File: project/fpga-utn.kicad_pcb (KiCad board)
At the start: 2 copper layers, 100 x 75 mm, 144 parts, among them J1 USB_C_Receptacle_USB2.0_16P, P1 Conector SMD 2x10, P2 Conector SMD 2x10, P3 Conector SMD 2x10, P4 Conector SMD 2x10, SW1 SW_Push, SW2 SW_Push, SW3 SW_Push, SW4 SW_Push, SW5 SW_Push, SW6 SW_Push, SW7 SW_Push, SW8 SW_Push, U1 LD1117S33TR_SOT223, U2 LD1117S12TR_SOT223, U3 USBLC6-2SC6, U4 FT2232HL, U5 M93C66, U6 ICE40HX4K-TQ144, U7 W25X40CLSN, Y1 ECS-3225MV-120-CN-TR, Y2 ECS-3225MVQ-1000-CN-TR

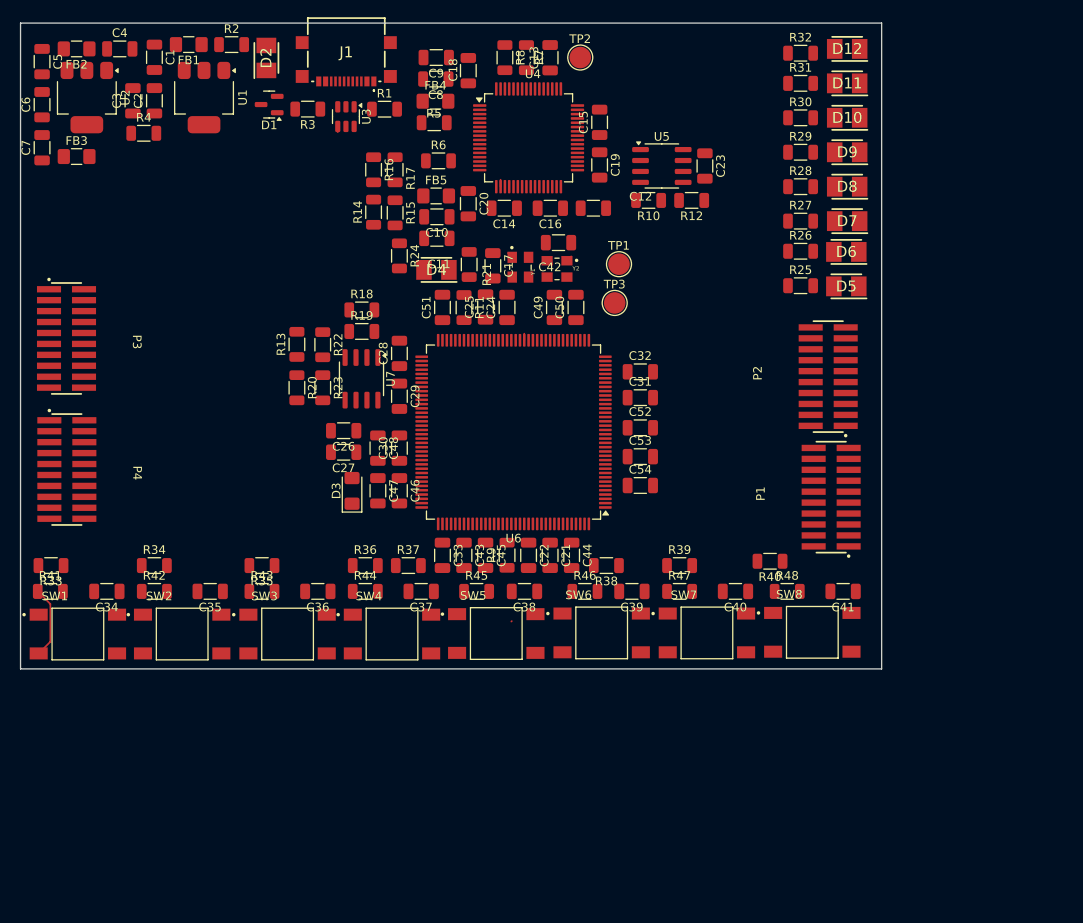
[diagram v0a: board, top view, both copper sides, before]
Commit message: Version 1 pcb, sin finalizar
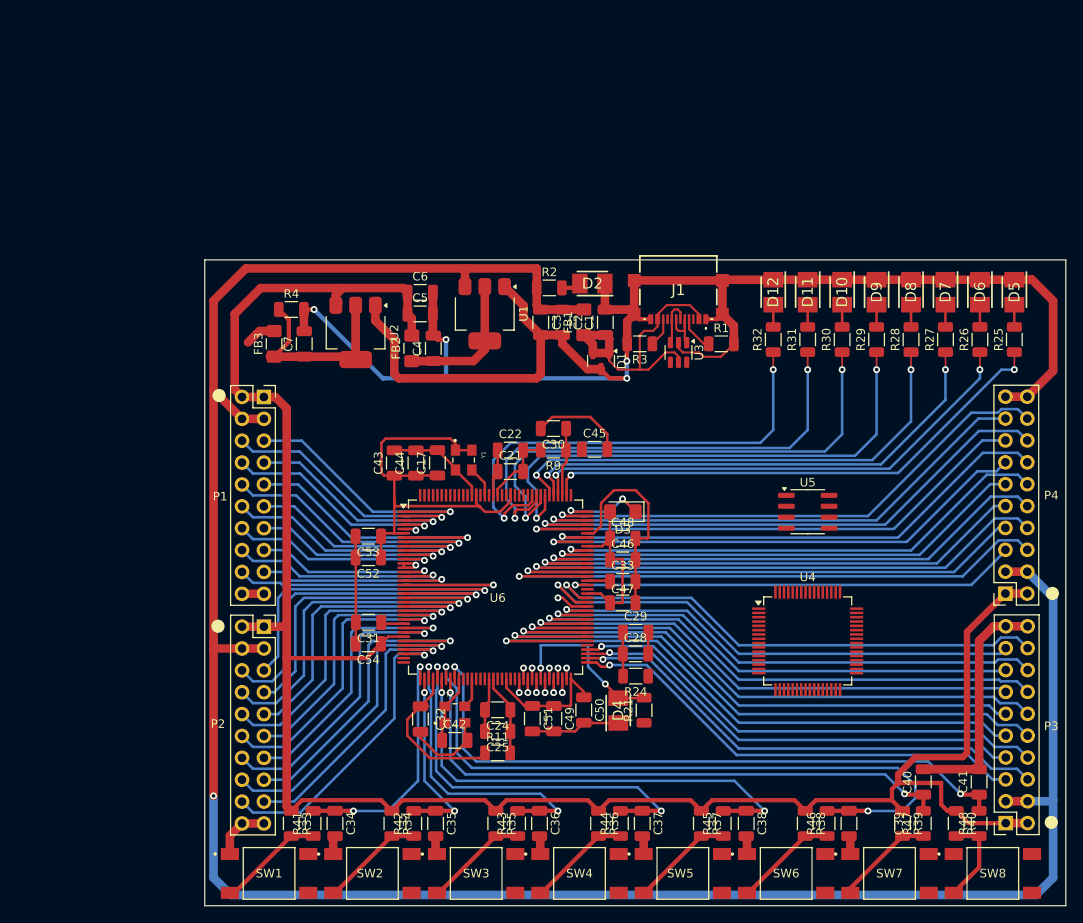
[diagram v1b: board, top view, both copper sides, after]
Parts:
- removed C10, C13, C14, C15, C16, C18, C19, C20, C23, C8: 100n, Capacitor_SMD:C_1206_3216Metric
- removed C11, C9: 4u7, Capacitor_SMD:C_1206_3216Metric
- removed C12: 3u3, Capacitor_SMD:C_1206_3216Metric
- removed C26: 10n, Capacitor_SMD:C_1206_3216Metric
- removed C27: 1u, Capacitor_SMD:C_1206_3216Metric
- removed FB4, FB5: FerriteBead_Small, Inductor_SMD:L_1206_3216Metric_Pad1.42x1.75mm_HandSolder
- removed R10: 2k2, Resistor_SMD:R_1206_3216Metric
- removed R12, R13, R19, R20, R7, R8: 10k, Resistor_SMD:R_1206_3216Metric
- removed R14, R22, R23: 220, Resistor_SMD:R_1206_3216Metric
- removed R15, R16, R17, R18: R, Resistor_SMD:R_1206_3216Metric
- removed R5: 12k, Resistor_SMD:R_1206_3216Metric
- removed R6: 1k, Resistor_SMD:R_1206_3216Metric
- removed TP1: 12MHZ, TestPoint:TestPoint_Pad_D2.5mm
- removed TP2: TP_PWR_EN, TestPoint:TestPoint_Pad_D2.5mm
- removed TP3: 100MHZ, TestPoint:TestPoint_Pad_D2.5mm
- removed U7: W25X40CLSN, Package_SO:SOIC-8_3.9x4.9mm_P1.27mm
- P1, P2, P3, P4: footprint FRT-FPGA:Header 2x10 SMD -> Connector_PinSocket_2.54mm:PinSocket_2x10_P2.54mm_Vertical
- moved P3 122.5 mm to (219.5, 139.7), turned to 180 degrees
- moved P4 109.7 mm to (219.5, 113.0), turned to 180 degrees
- moved P2 71.5 mm to (133.3, 116.8), turned to 0 degrees
- moved U4 66.8 mm to (196.5, 118.5)
- moved P1 66.6 mm to (133.3, 90.2), turned to 0 degrees
- moved C1 60.7 mm to (173.0, 81.5), turned to 90 degrees
- moved C42 59.0 mm to (155.5, 130.1), turned to 0 degrees
- moved FB1 56.1 mm to (170.5, 81.5), turned to 90 degrees
- moved R24 56.0 mm to (176.5, 122.6), turned to 180 degrees
- moved R21 55.6 mm to (177.5, 126.5), turned to 90 degrees
- moved D4 55.4 mm to (174.5, 126.6), turned to 90 degrees
- moved C2 53.9 mm to (168.0, 81.5), turned to -90 degrees
- moved C3 53.9 mm to (165.5, 81.5), turned to -90 degrees
- moved Y2 53.1 mm to (155.5, 127.0), turned to 0 degrees
- moved C5 52.8 mm to (151.5, 80.5), turned to 0 degrees
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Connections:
- U6 pad 1: Net-(U6D-IOL_2A) -> Net-(P1-IO1)
- U6 pad 10: Net-(U6D-IOL_5B) -> Net-(P1-IO8)
- U6 pad 101: Net-(U6B-IOR_160) -> Net-(P4-IO9)
- U6 pad 102: Net-(U6B-IOR_161) -> Net-(P4-IO10)
- U6 pad 104: Net-(U6B-IOR_164) -> Net-(P4-IO11)
- U6 pad 105: Net-(U6B-IOR_165) -> Net-(P4-IO12)
- U6 pad 106: Net-(U6B-IOR_166) -> Net-(P4-IO13)
- U6 pad 107: Net-(U6B-IOR_167) -> Net-(P4-IO14)
- U6 pad 11: Net-(U6D-IOL_8A) -> Net-(P1-IO9)
- U6 pad 110: unconnected-(U6A-IOT_168-Pad110) -> /Perifericos/LED1
- U6 pad 112: unconnected-(U6A-IOT_169-Pad112) -> /Perifericos/LED2
- U6 pad 113: unconnected-(U6A-IOT_170-Pad113) -> /Perifericos/LED3
- U6 pad 114: unconnected-(U6A-IOT_171-Pad114) -> /Perifericos/LED4
- U6 pad 115: unconnected-(U6A-IOT_172-Pad115) -> /Perifericos/LED5
- U6 pad 116: unconnected-(U6A-IOT_173-Pad116) -> /Perifericos/LED6
- U6 pad 117: unconnected-(U6A-IOT_174-Pad117) -> /Perifericos/LED7
- U6 pad 118: unconnected-(U6A-IOT_177-Pad118) -> /Perifericos/LED8
- U6 pad 12: Net-(U6D-IOL_8B) -> Net-(P1-IO10)
- U6 pad 129: unconnected-(U6A-IOT_198_GBIN0-Pad129) -> /Perifericos/12MHz_CLK
- U6 pad 136: /Perifericos/BOT8 -> unconnected-(U6A-IOT_214-Pad136)
- U6 pad 137: /Perifericos/BOT7 -> unconnected-(U6A-IOT_215-Pad137)
- U6 pad 138: /Perifericos/BOT6 -> unconnected-(U6A-IOT_216-Pad138)
- U6 pad 139: /Perifericos/BOT5 -> unconnected-(U6A-IOT_217-Pad139)
- U6 pad 141: /Perifericos/BOT4 -> unconnected-(U6A-IOT_219-Pad141)
- U6 pad 142: /Perifericos/BOT3 -> unconnected-(U6A-IOT_220-Pad142)
- U6 pad 143: /Perifericos/BOT2 -> unconnected-(U6A-IOT_221-Pad143)
- U6 pad 144: /Perifericos/BOT1 -> unconnected-(U6A-IOT_222-Pad144)
- U6 pad 15: Net-(U6D-IOL_10A) -> Net-(P1-IO11)
- U6 pad 16: Net-(U6D-IOL_10B) -> Net-(P1-IO12)
- U6 pad 17: Net-(U6D-IOL_12A) -> Net-(P1-IO13)
- U6 pad 18: Net-(U6D-IOL_12B) -> Net-(P1-IO14)
- U6 pad 19: Net-(U6D-IOL_13A) -> Net-(P2-IO1)
- U6 pad 2: Net-(U6D-IOL_2B) -> Net-(P1-IO2)
- U6 pad 20: Net-(U6D-IOL_13B_GBIN7) -> Net-(P2-IO2)
- U6 pad 21: Net-(U6D-IOL_14A_GBIN6) -> Net-(P2-IO3)
- U6 pad 22: Net-(U6D-IOL_14B) -> Net-(P2-IO4)
- U6 pad 23: Net-(U6D-IOL_17A) -> Net-(P2-IO5)
- U6 pad 24: Net-(U6D-IOL_17B) -> Net-(P2-IO6)
- U6 pad 25: Net-(U6D-IOL_18A) -> Net-(P2-IO7)
- U6 pad 26: Net-(U6D-IOL_18B) -> Net-(P2-IO8)
- U6 pad 28: Net-(U6D-IOL_23A) -> Net-(P2-IO9)
- U6 pad 29: Net-(U6D-IOL_23B) -> Net-(P2-IO10)
- U6 pad 3: Net-(U6D-IOL_3A) -> Net-(P1-IO3)
- U6 pad 31: Net-(U6D-IOL_24A) -> Net-(P2-IO11)
- U6 pad 32: Net-(U6D-IOL_24B) -> Net-(P2-IO12)
- U6 pad 33: Net-(U6D-IOL_25A) -> Net-(P2-IO13)
- U6 pad 34: Net-(U6D-IOL_25B) -> Net-(P2-IO14)
- U6 pad 37: /Perifericos/LED1 -> /Perifericos/BOT1
- U6 pad 38: /Perifericos/LED2 -> /Perifericos/BOT2
- U6 pad 39: /Perifericos/LED3 -> /Perifericos/BOT3
- U6 pad 4: Net-(U6D-IOL_3B) -> Net-(P1-IO4)
- U6 pad 41: /Perifericos/LED4 -> /Perifericos/BOT4
- U6 pad 42: /Perifericos/LED5 -> /Perifericos/BOT5
- U6 pad 43: /Perifericos/LED6 -> /Perifericos/BOT6
- U6 pad 44: /Perifericos/LED7 -> /Perifericos/BOT7
- U6 pad 45: /Perifericos/LED8 -> /Perifericos/BOT8
- U6 pad 52: /Perifericos/12MHz_CLK -> unconnected-(U6C-IOB_82_GBIN4-Pad52)
- U6 pad 7: Net-(U6D-IOL_4A) -> Net-(P1-IO5)
- U6 pad 73: Net-(U6B-IOR_109) -> Net-(P3-IO1)
- U6 pad 74: Net-(U6B-IOR_110) -> Net-(P3-IO2)
- U6 pad 75: Net-(U6B-IOR_111) -> Net-(P3-IO3)
- U6 pad 76: Net-(U6B-IOR_112) -> Net-(P3-IO4)
- U6 pad 78: Net-(U6B-IOR_114) -> Net-(P3-IO5)
- U6 pad 79: Net-(U6B-IOR_115) -> Net-(P3-IO6)
- U6 pad 8: Net-(U6D-IOL_4B) -> Net-(P1-IO6)
- U6 pad 80: Net-(U6B-IOR_116) -> Net-(P3-IO7)
- U6 pad 81: Net-(U6B-IOR_117) -> Net-(P3-IO8)
- U6 pad 82: Net-(U6B-IOR_118) -> Net-(P3-IO9)
- U6 pad 83: Net-(U6B-IOR_119) -> Net-(P3-IO10)
- U6 pad 84: Net-(U6B-IOR_120) -> Net-(P3-IO11)
- U6 pad 85: Net-(U6B-IOR_128) -> Net-(P3-IO12)
- U6 pad 87: Net-(U6B-IOR_136) -> Net-(P3-IO13)
- U6 pad 88: Net-(U6B-IOR_137) -> Net-(P3-IO14)
- U6 pad 9: Net-(U6D-IOL_5A) -> Net-(P1-IO7)
- U6 pad 91: Net-(U6B-IOR_139) -> Net-(P4-IO1)
- U6 pad 93: Net-(U6B-IOR_140_GBIN3) -> Net-(P4-IO2)
- U6 pad 94: Net-(U6B-IOR_141_GBIN2) -> Net-(P4-IO3)
- U6 pad 95: Net-(U6B-IOR_144) -> Net-(P4-IO4)
- U6 pad 96: Net-(U6B-IOR_146) -> Net-(P4-IO5)
- U6 pad 97: Net-(U6B-IOR_147) -> Net-(P4-IO6)
- U6 pad 98: Net-(U6B-IOR_148) -> Net-(P4-IO7)
- U6 pad 99: Net-(U6B-IOR_152) -> Net-(P4-IO8)
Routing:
- net GND: track 0.51 -> 351.6 mm, vias 0 -> 8
- net +3V3: track 1.40 -> 344.0 mm
- net +5V: track 0.00 -> 275.3 mm, vias 0 -> 1
- net /Perifericos/BOT6: track 0.00 -> 79.1 mm, vias 0 -> 2
- net /Perifericos/BOT8: track 0.00 -> 75.3 mm, vias 0 -> 2
- net Net-(P3-IO6): track 0.00 -> 72.8 mm, vias 0 -> 1
- net Net-(P3-IO5): track 0.00 -> 72.0 mm, vias 0 -> 1
- net Net-(P4-IO2): track 0.00 -> 69.1 mm, vias 0 -> 1
- net Net-(P3-IO8): track 0.00 -> 68.2 mm, vias 0 -> 1
- net /Perifericos/BOT7: track 0.00 -> 67.9 mm, vias 0 -> 2
- net Net-(P3-IO7): track 0.00 -> 67.5 mm, vias 0 -> 1
- net Net-(P4-IO12): track 0.00 -> 66.0 mm, vias 0 -> 1
- net Net-(P4-IO4): track 0.00 -> 65.9 mm, vias 0 -> 1
- net Net-(P4-IO11): track 0.00 -> 64.6 mm, vias 0 -> 1
- net Net-(P4-IO3): track 0.00 -> 64.6 mm, vias 0 -> 1
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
